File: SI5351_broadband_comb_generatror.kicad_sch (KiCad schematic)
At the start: 8 parts, among them J1 Conn_Coaxial_Small, J3 Barrel_Jack_Switch, J4 Conn_Coaxial_Small, J9 Conn_Coaxial_Small

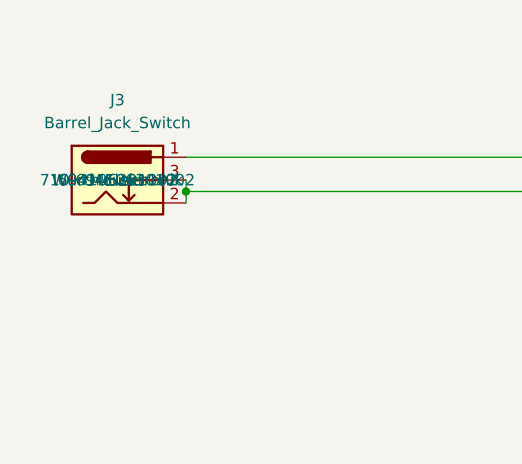
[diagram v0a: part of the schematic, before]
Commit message: BOM...
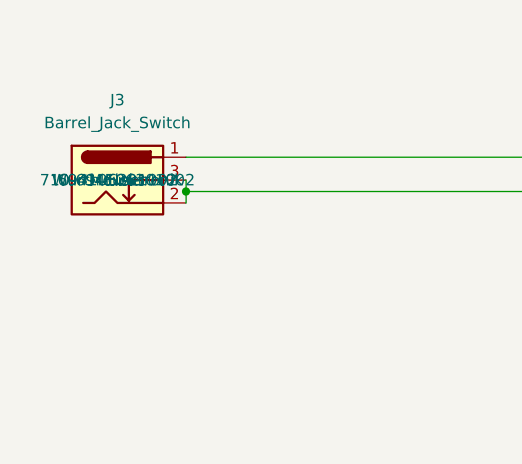
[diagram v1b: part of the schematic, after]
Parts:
- J3: Manufacturer Würth Elektronik -> Wurth Elektronik
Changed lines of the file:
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@@
 			)
 		)
-		(property "Manufacturer" "Würth Elektronik"
+		(property "Manufacturer" "Wurth Elektronik"
 			(at 68.58 53.34 0)
 			(effects
